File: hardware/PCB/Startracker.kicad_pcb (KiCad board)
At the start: 4 copper layers, 99.8 x 99.8 mm, 135 parts, among them IC1 BNO085, IC2 IIS2MDCTR, J1 IMU_EXT, J2 GPS, J3 Motor1, J4 Motor2, J5 Motor3, J6 6V, J7 SJ-3523-SMT-TR, J8 USB_C_Receptacle_USB2.0_16P, Q1 2N3904, Q2 2N3904, SW1 RST, SW2 BOOT, SW3 PWR, U1 ESP32-S3-WROOM-1, U10 SX1261IMLTRT, U11 BGS12P2L6E6327XT, U12 SRV05-4, U13 TPS54308, U14 TPS2121RUXR, U2 TMC2209-LA, U3 TB6612FNG, U4 TB6612FNG, U5 PCF8574T, U7 BME280, U8 INA219BxDCN, U9 INA219BxDCN, Y1 Crystal, Y2 32.00 MHz

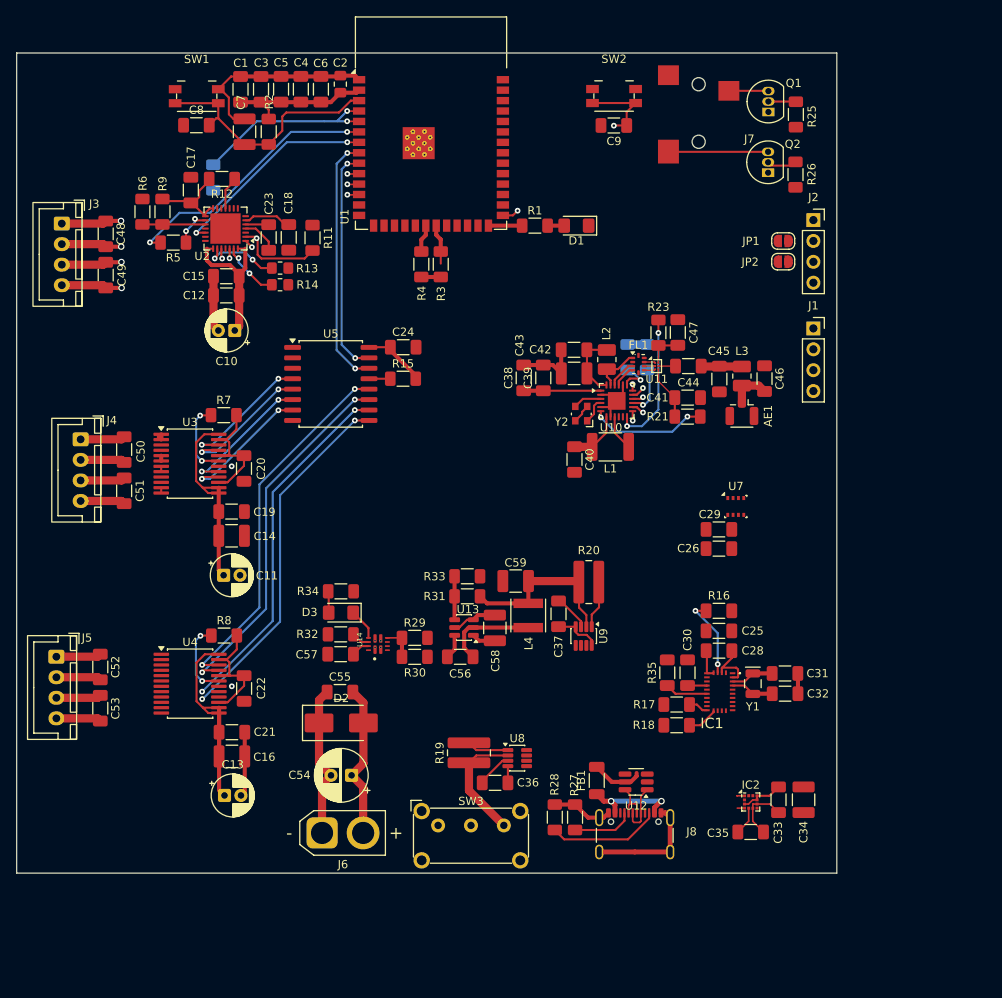
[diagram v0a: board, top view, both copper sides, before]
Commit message: Finished routing and layout of PCB
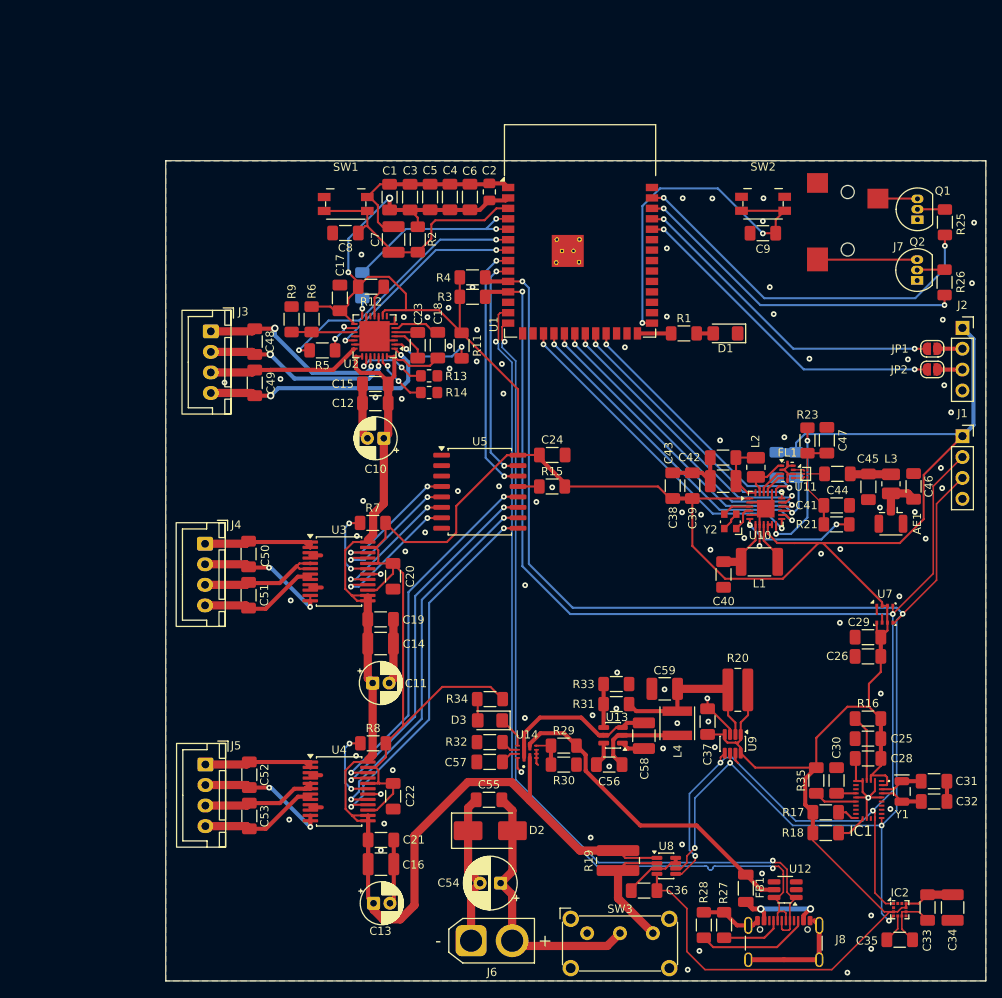
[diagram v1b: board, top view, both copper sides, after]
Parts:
- U1: footprint RF_Module:ESP32-S3-WROOM-1 -> saját:sa
- moved R6 24.4 mm to (108.9, 68.4), turned to 90 degrees
- moved L1 22.9 mm to (163.4, 97.9)
- moved C40 22.9 mm to (159.1, 99.4)
- moved C13 22.4 mm to (116.5, 139.4)
- moved C26 22.4 mm to (176.6, 109.4)
- moved C35 22.4 mm to (180.5, 143.9)
- moved C36 22.4 mm to (149.4, 137.9)
- moved C37 22.4 mm to (157.1, 117.3)
- moved C41 22.4 mm to (172.8, 91.0)
- moved C59 22.4 mm to (151.9, 113.4)
- moved FB1 22.4 mm to (161.8, 137.6)
- moved JP1 22.4 mm to (184.5, 72.0)
- moved R11 22.4 mm to (127.2, 71.6)
- moved R17 22.4 mm to (171.5, 128.4)
- moved R19 22.4 mm to (146.2, 134.2)
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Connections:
- C26 pad 1: GND_1 -> GND
- C29 pad 1: GND_1 -> GND
- C33 pad 1: GND_1 -> GND
- C34 pad 1: GND_1 -> GND
- C35 pad 2: GND_1 -> GND
- C36 pad 1: GND_1 -> GND
- C37 pad 1: GND_1 -> GND
- IC2 pad 6: GND_1 -> GND
- IC2 pad 8: GND_1 -> GND
- R3 pad 1: /OBC/I2C_SDA -> /OBC/I2C_SCL
- R4 pad 1: /OBC/I2C_SCL -> /OBC/I2C_SDA
- U1 pad 10: /OBC/I2C_SCL -> /OBC/I2C_SDA
- U1 pad 11: /OBC/I2C_SDA -> /OBC/I2C_SCL
- U1 pad 17: /LORA/SX_RST -> /LORA/SX_DIO1
- U1 pad 18: /LORA/SX_SCK -> /LORA/SX_BUSY
- U1 pad 19: /LORA/SX_MOSI -> /LORA/SX_RST
- U1 pad 21: /LORA/SX_NSS -> /LORA/SX_MOSI
- U1 pad 22: /LORA/SX_DIO1 -> /LORA/SX_SCK
- U1 pad 23: /LORA/SX_BUSY -> /LORA/SX_NSS
- U7 pad 1: GND_1 -> GND
- U7 pad 7: GND_1 -> GND
- U8 pad 3: GND_1 -> GND
- U8 pad 7: GND_1 -> GND
- U8 pad 8: GND_1 -> GND
- U9 pad 3: GND_1 -> GND
- U9 pad 7: GND_1 -> GND
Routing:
- net +3.3V: track 110.1 -> 458.6 mm, vias 0 -> 2
- net /OBC/I2C_SCL: track 5.72 -> 187.9 mm, vias 1 -> 5
- net /OBC/I2C_SDA: track 7.15 -> 188.0 mm, vias 1 -> 6
- net /OBC/USB_D-: track 5.06 -> 106.3 mm, vias 0 -> 2
- net /OBC/USB_D+: track 6.25 -> 105.3 mm, vias 0 -> 2
- net VM: track 77.6 -> 163.8 mm
- net GND: track 107.3 -> 187.7 mm, vias 2 -> 88
- net /CONN/Focus: track 0.00 -> 46.1 mm, vias 0 -> 2
- net /CONN/Shutter: track 0.00 -> 41.7 mm, vias 0 -> 2
- net /OBC/GPS_RX: track 0.00 -> 40.6 mm, vias 0 -> 2
- net /OBC/GPS_TX: track 0.00 -> 40.0 mm, vias 0 -> 2
- net /LORA/SX_DIO1: track 1.12 -> 40.7 mm, vias 1 -> 2
- net /LORA/SX_BUSY: track 1.42 -> 40.6 mm, vias 1 -> 2
- net /LORA/SX_RST: track 6.03 -> 43.5 mm, vias 1 -> 2
- net /LORA/SX_MISO: track 1.21 -> 37.1 mm, vias 1 -> 2
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- added copper zone on B.Cu, net GND
- added copper zone on F.Cu, net GND
- added copper zone on In1.Cu, net GND
- added copper zone on In2.Cu, net GND
